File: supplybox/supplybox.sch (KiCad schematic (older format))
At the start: 12 parts, among them J1 Screw_Terminal_01x02

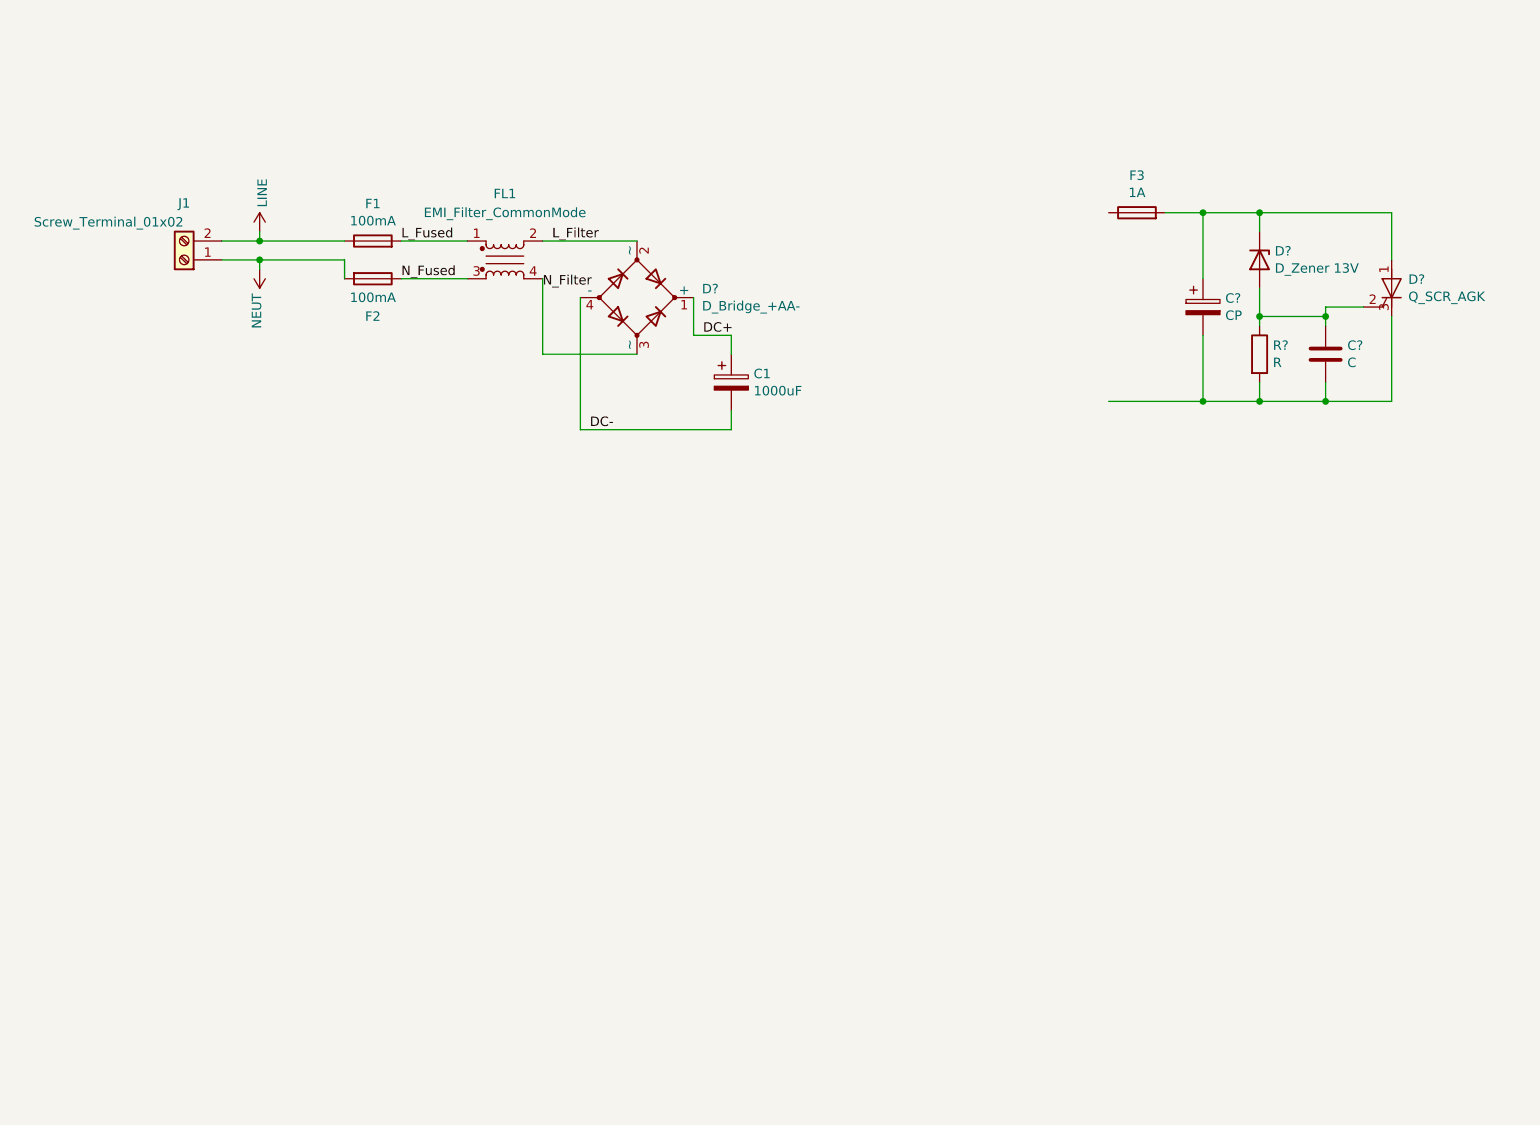
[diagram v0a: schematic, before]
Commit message: v1.0
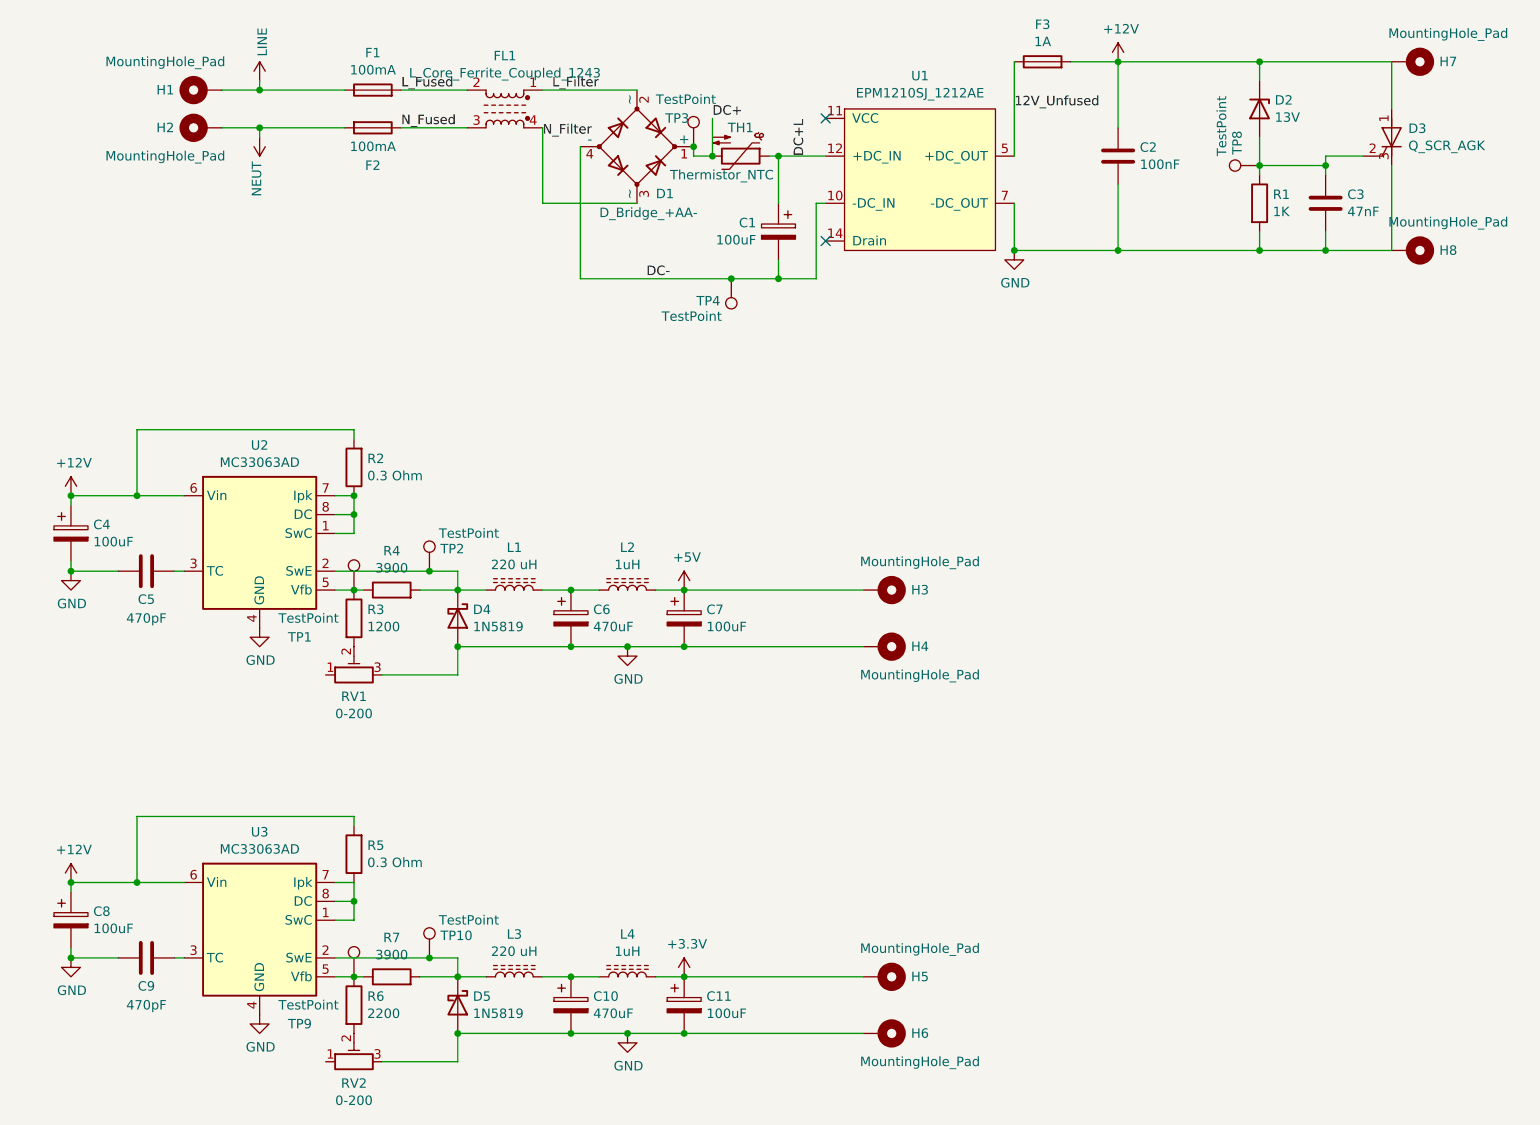
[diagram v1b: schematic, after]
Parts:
- removed C?: CP, symbol Device:CP
- removed FL1: EMI_Filter_CommonMode, Inductor_THT:L_CommonMode_Wuerth_WE-CMB-XS, symbol Device:EMI_Filter_CommonMode
- removed J1: Screw_Terminal_01x02, symbol Connector:Screw_Terminal_01x02
- added C10, C6: 470uF, Capacitor_THT:CP_Radial_D8.0mm_P3.50mm, symbol Device:CP
- added C11, C4, C7, C8: 100uF, Capacitor_THT:CP_Radial_D6.3mm_P2.50mm, symbol Device:CP
- added C2: 100nF, Capacitor_SMD:C_0603_1608Metric_Pad1.05x0.95mm_HandSolder, symbol Device:C
- added C5, C9: 470pF, Capacitor_SMD:C_0603_1608Metric_Pad1.05x0.95mm_HandSolder, symbol Device:C
- added D4, D5: 1N5819, Diode_THT:D_DO-41_SOD81_P10.16mm_Horizontal, symbol Diode:1N5819
- added FL1: L_Core_Ferrite_Coupled_1243, Inductor_THT:L_CommonMode_Wuerth_WE-CMB-XS, symbol Device:L_Core_Ferrite_Coupled_1243
- added H1, H2, H3, H4, H5, H6, H7, H8: MountingHole_Pad, MountingHole:MountingHole_3.2mm_M3_DIN965_Pad, symbol Mechanical:MountingHole_Pad
- added L1, L3: 220 uH, Inductor_THT:L_Radial_D9.5mm_P5.00mm_Fastron_07HVP, symbol Device:L_Core_Ferrite
- added L2, L4: 1uH, Inductor_SMD:L_0805_2012Metric_Pad1.15x1.40mm_HandSolder, symbol Device:L_Core_Ferrite
- added R2, R5: 0.3 Ohm, Resistor_SMD:R_0805_2012Metric_Pad1.15x1.40mm_HandSolder, symbol Device:R
- added R3: 1200, Resistor_SMD:R_0603_1608Metric_Pad1.05x0.95mm_HandSolder, symbol Device:R
- added R4, R7: 3900, Resistor_SMD:R_0603_1608Metric_Pad1.05x0.95mm_HandSolder, symbol Device:R
- added R6: 2200, Resistor_SMD:R_0603_1608Metric_Pad1.05x0.95mm_HandSolder, symbol Device:R
- added RV1, RV2: 0-200, Potentiometer_SMD:Potentiometer_Bourns_TC33X_Vertical, symbol Device:R_POT_TRIM
- added TH1: Thermistor_NTC, Resistor_THT:R_Axial_DIN0204_L3.6mm_D1.6mm_P5.08mm_Horizontal, symbol Device:Thermistor_NTC
- added TP1, TP10, TP2, TP3, TP4, TP8, TP9: TestPoint, TestPoint:TestPoint_Pad_D1.0mm, symbol Connector:TestPoint
- added U1: EPM1210SJ_1212AE, ERIG_Converter_DCDC:EPMXX10SJ_XXXXAE, symbol ERIG_Converter_DCDC:EPM1210SJ_1212AE
- added U2, U3: MC33063AD, Package_SO:SOIC-8_3.9x4.9mm_P1.27mm, symbol Regulator_Switching:MC33063AD
- C1: value 1000uF -> 100uF; footprint (none) -> Capacitor_THT:CP_Radial_D18.0mm_P7.50mm; digikey (none) -> 565-1481-ND
- C3: renamed from C?; value C -> 47nF; footprint (none) -> Capacitor_SMD:C_0603_1608Metric_Pad1.05x0.95mm_HandSolder; digikey (none) -> 1292-1446-1-ND
- D1: renamed from D?; footprint (none) -> ERIG_Diode:KBP20XXG; digikey (none) -> KBP206GDI-ND
- D2: renamed from D?; value D_Zener 13V -> 13V; footprint (none) -> Diode_SMD:D_SOT-23_ANK; digikey (none) -> BZX84C13LT1GOSCT-ND
- D3: renamed from D?; footprint (none) -> Package_TO_SOT_THT:TO-92; digikey (none) -> 1740-1089-1-ND
- F1, F2: footprint (none) -> ERIG_Fuse:RST_XXX; digikey RST100AMMO-ND -> 507-1166-ND
- F3: footprint (none) -> Fuse:Fuse_0805_2012Metric_Pad1.15x1.40mm_HandSolder; digikey (none) -> MFU08051.00CT-ND
- R1: renamed from R?; value R -> 1K; footprint (none) -> Resistor_SMD:R_0603_1608Metric_Pad1.05x0.95mm_HandSolder; digikey (none) -> RHM1.0KDCT-ND
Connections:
- net labels added: +12V, +3.3V, +5V, 12V_Unfused, DC+L, GND
- wire segments 38 -> 108
- no-connect marks 0 -> 2
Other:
- moved on the sheet: C1, C3, D1, D2, D3, F1, F2, F3, R1
